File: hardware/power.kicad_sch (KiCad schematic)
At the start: 16 parts, among them Q3 DMG1012T, U2 MAX20049ATED/VY+

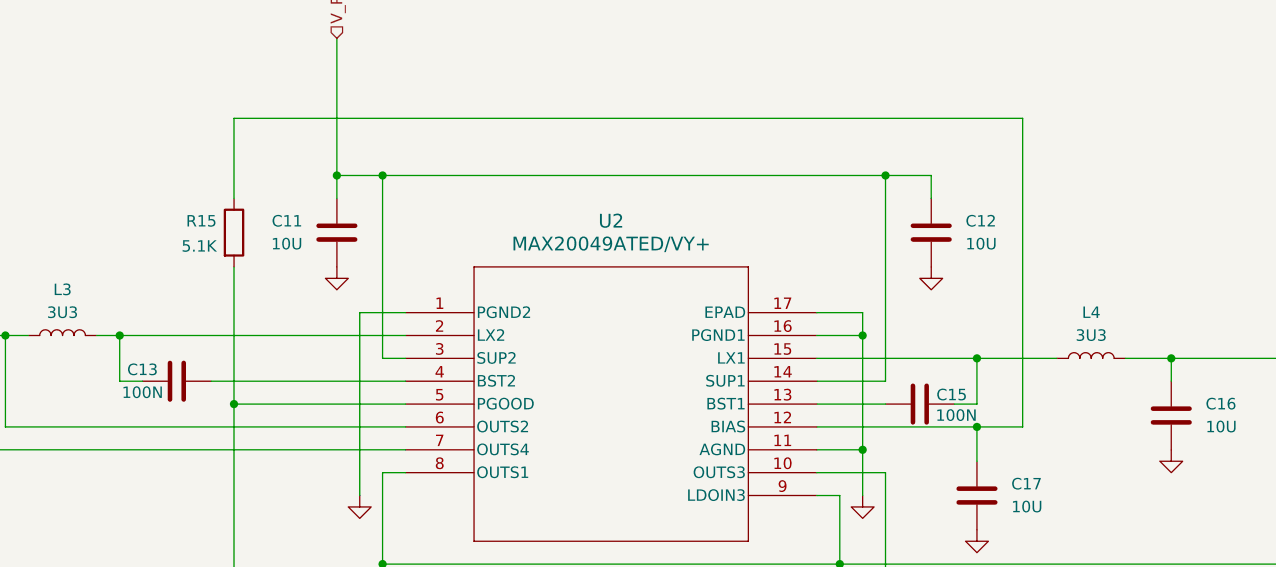
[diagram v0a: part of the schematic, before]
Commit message: prepping for fab
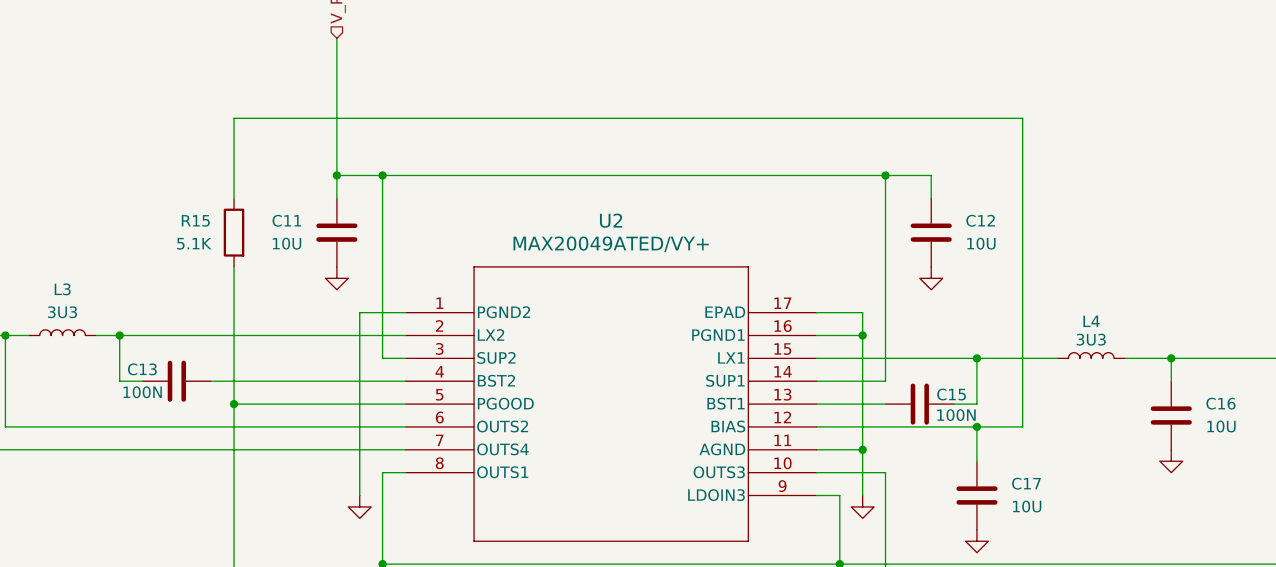
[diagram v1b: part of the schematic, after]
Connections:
- net +3V3: now also L4.1; no longer L4.2
- net at C15.2, U2.15 (LX1): now also L4.2; no longer L4.1
